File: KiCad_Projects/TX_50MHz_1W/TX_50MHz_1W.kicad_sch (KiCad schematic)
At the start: 38 parts, among them J1 AIL Stick, J10 I2C Exp / OLED, J11 ANT, J2 ELE Stick, J3 THR Stick, J4 RUD Stick, J5 AUX5, J6 AUX6, J7 AUX7, J8 V_BATT In (XT30), J9 5V Logic In, Q1 RD01MUS2 (1W PA), U1 ESP32-S3-WROOM-1-N16R8, U2 Si5351A-B-GT, U3 BGS12PL6 (T/R SW), U4 SPF5043Z (LNA), U5 LT5560 (Mixer), U6 ADS1115IDGSR (0x48), U7 ADS1115IDGSR (0x49), U8 SH1106 1.3in OLED, Y1 26.000MHz

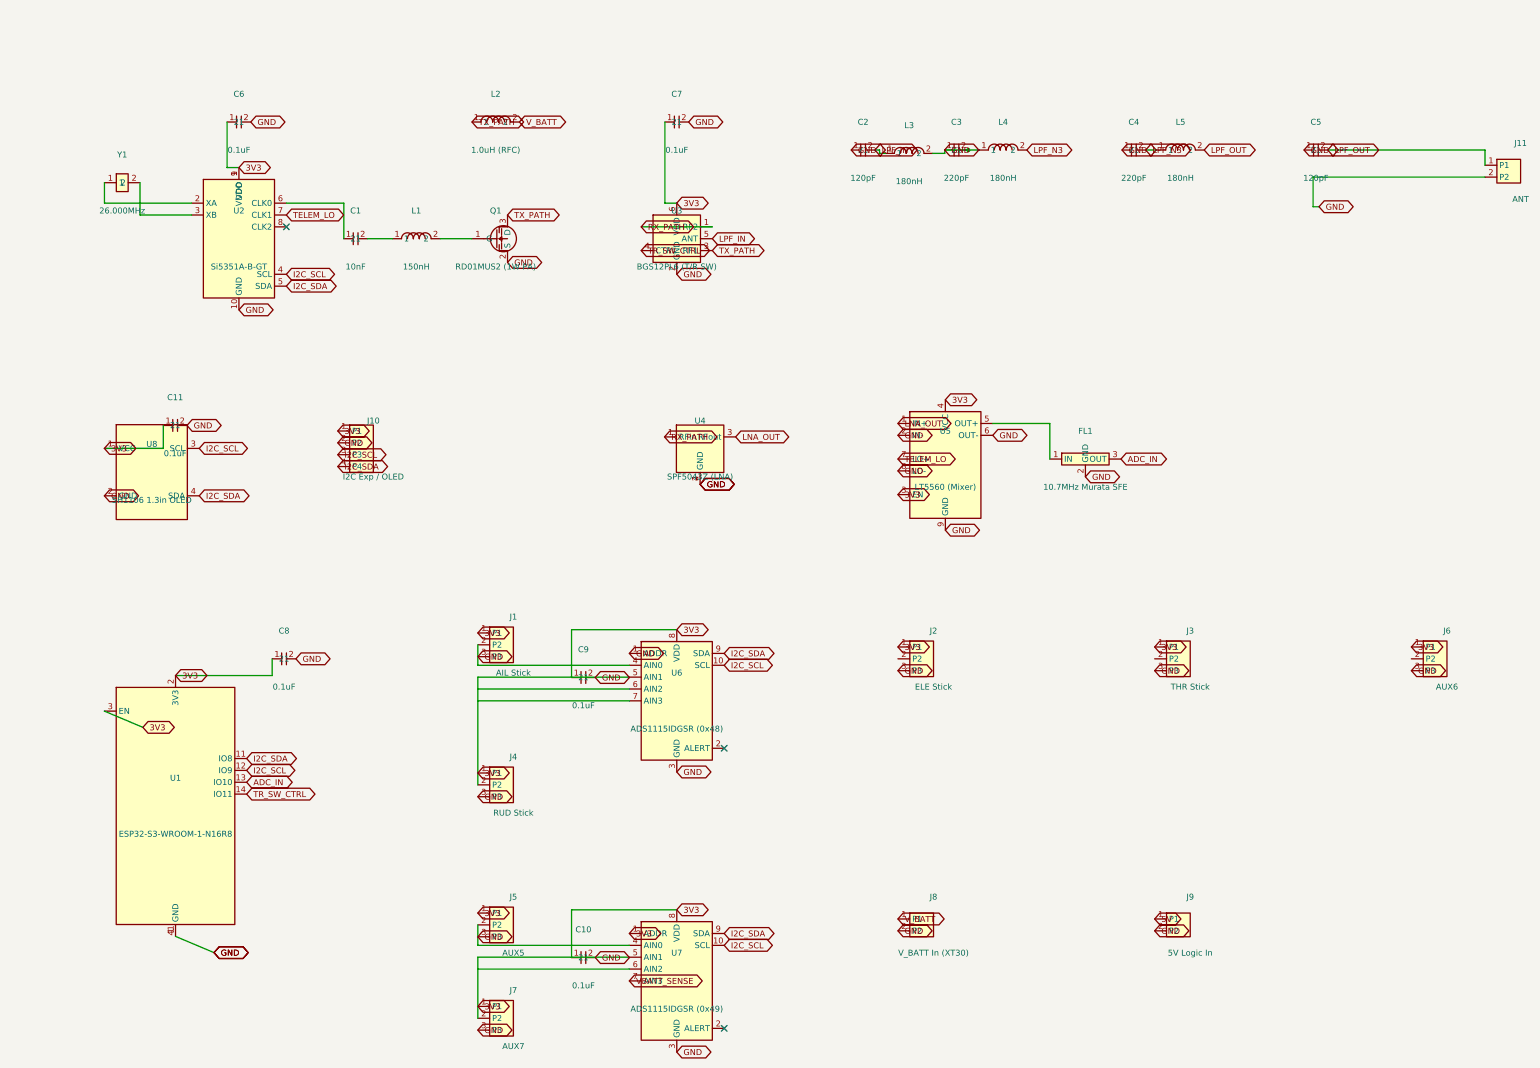
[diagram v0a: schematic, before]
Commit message: impove readabality
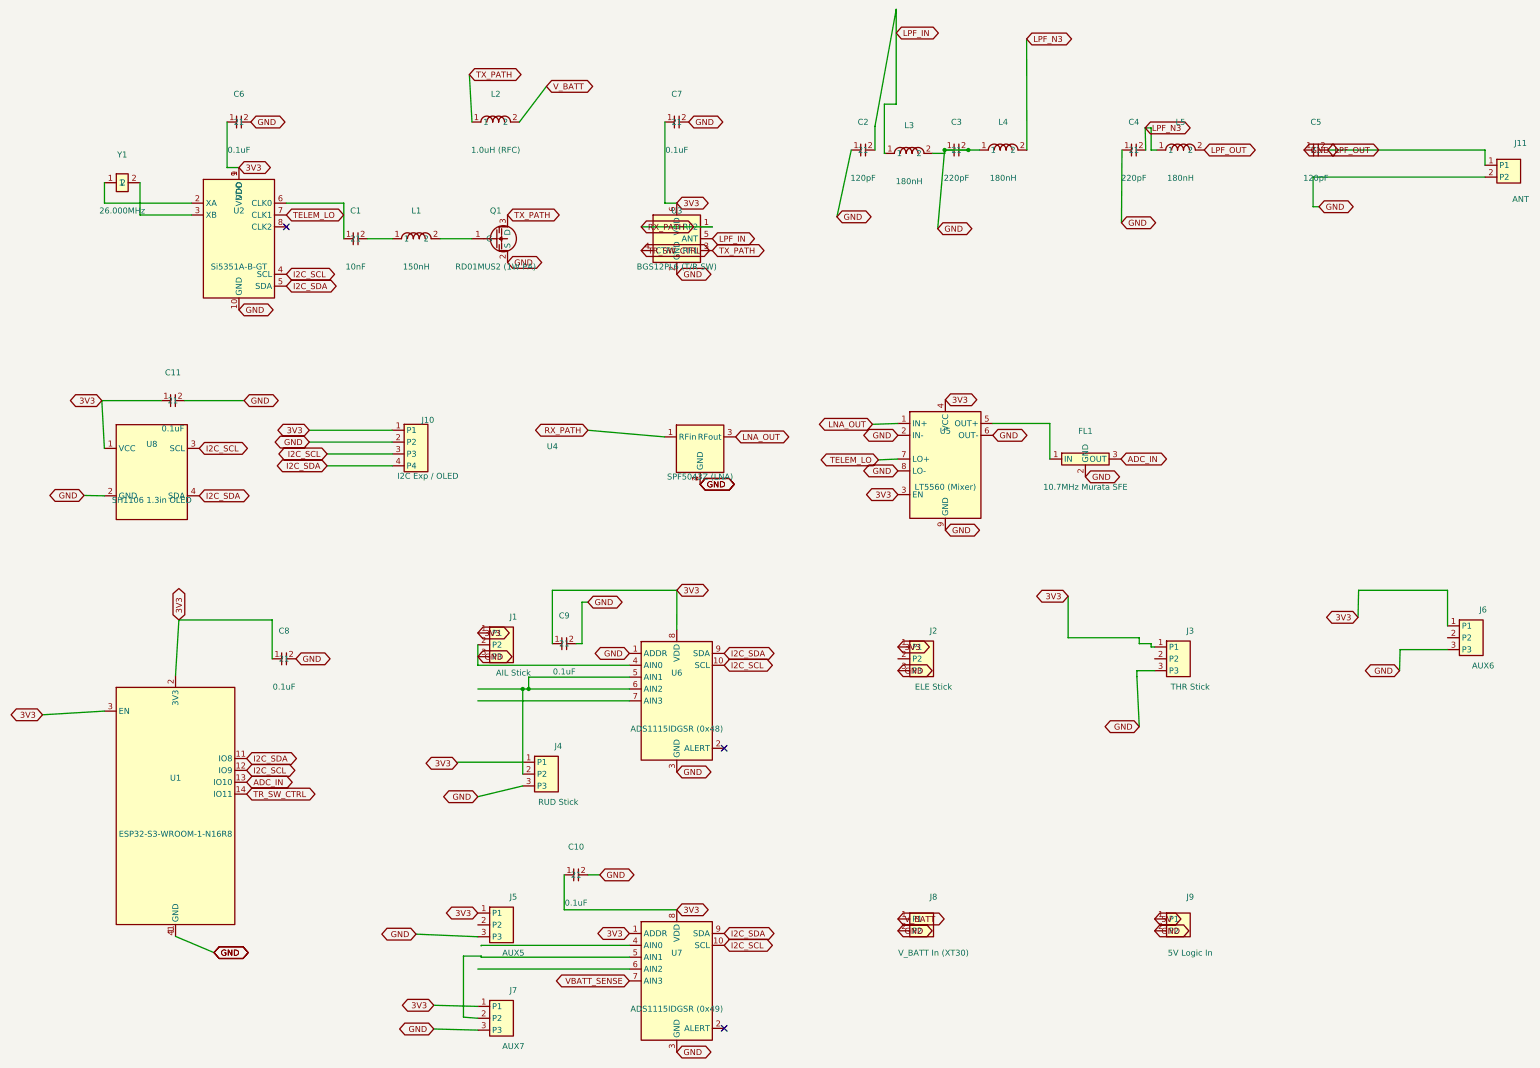
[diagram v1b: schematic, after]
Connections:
- net 3V3: no longer J4.1 (P1), J4.2 (P2), J7.2 (P2), U6.5 (AIN1), U7.5 (AIN1)
- net GND: now also C3.2, L3.2, L4.1; no longer J5.2 (P2), U7.4 (AIN0)
- net at U6.6 (AIN2): now also J4.2 (P2), U6.5 (AIN1)
- new net: J7.2 (P2), U7.5 (AIN1)
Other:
- moved on the sheet: C10, C11, C9, J10, J4, J6
